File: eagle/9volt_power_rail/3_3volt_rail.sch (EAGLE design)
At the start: 32 parts, among them X1 5566-4, X2 5566-4, X3 5566-4, X4 5566-4, X5 5566-4, X6 5566-4

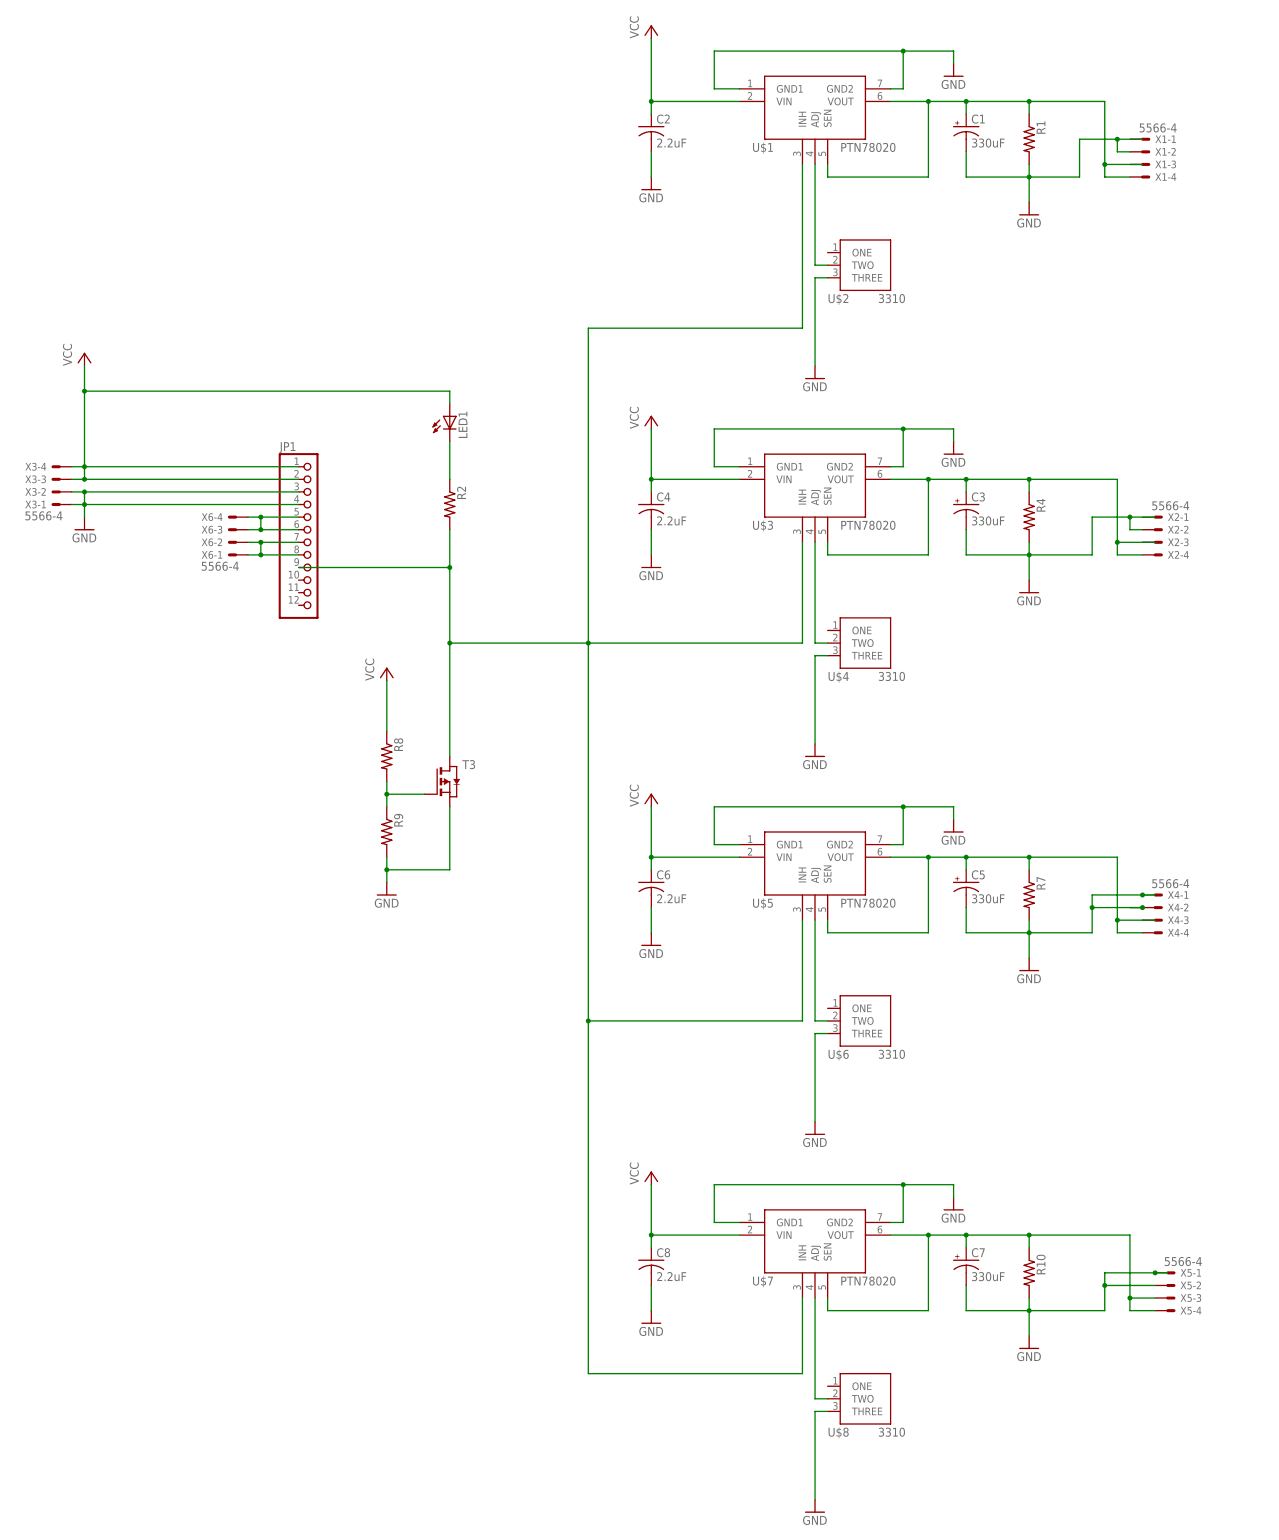
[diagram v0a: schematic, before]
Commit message: moving to lab computer
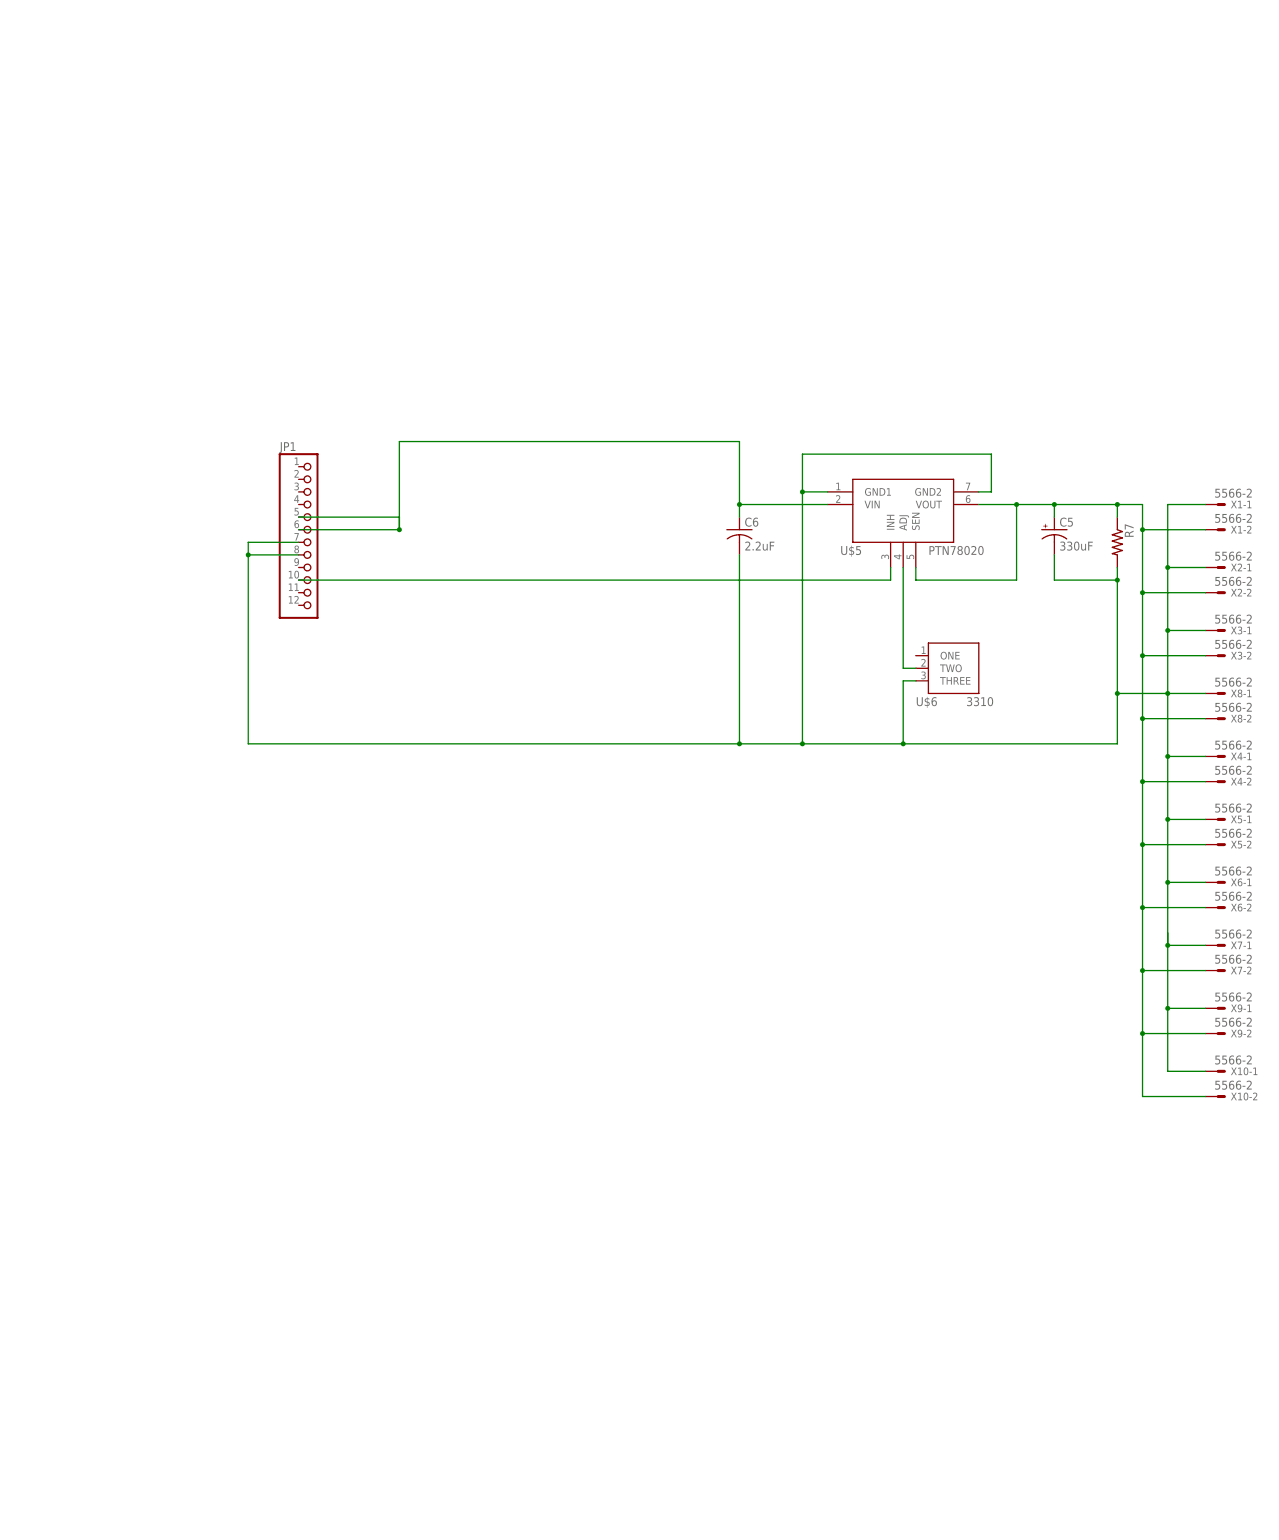
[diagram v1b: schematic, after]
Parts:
- removed C1, C3, C7: 330uF, rcl:CPOL-USE5-10.5
- removed C2, C4, C8: 2.2uF, adafruit:C-USC0805
- removed LED1: (no value), adafruit:LED5MM
- removed R1, R10, R2, R4, R8, R9: (no value), adafruit:R-US_M0805
- removed T3: (no value), zetex:PMOSSOT223
- removed U$1, U$3, U$7: PTH78020-SMD, PTN78020:PTH78020-SMD
- removed U$2, U$4, U$8: 3310-001, 3310-001:3310-001
- added X10, X7, X8, X9: 5566-2, con-molex:5566-2
- X1, X2, X3, X4, X5, X6: value 5566-4 -> 5566-2; device con-molex:5566-4 -> con-molex:5566-2
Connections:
- removed net GND: C1.-, C2.2, C3.-, C4.2, C5.-, C6.2, C7.-, C8.2, JP1.3, JP1.4, R1.2, R10.2, R4.2, R7.2, R9.2, T3.S, U$1.GND1, U$1.GND2, U$2.THREE, U$3.GND1, U$3.GND2, U$4.THREE, U$5.GND1, U$5.GND2, U$6.THREE, U$7.GND1, U$7.GND2, U$8.THREE, X1-2.S, X2-2.S, X3-1.S, X3-2.S, X4-1.S, X4-2.S, X5-1.S, X5-2.S
- removed net N$1: C3.+, R4.1, U$3.SEN, U$3.VOUT, X2-4.S
- removed net N$10: JP1.7, JP1.8, X6-1.S, X6-2.S
- removed net N$12: U$3.ADJ, U$4.TWO
- removed net N$14: R8.2, R9.1, T3.G
- removed net N$2: U$1.ADJ, U$2.TWO
- removed net N$22: U$7.ADJ, U$8.TWO
- removed net N$5: JP1.9, R2.2, T3.D, U$1.INH, U$3.INH, U$5.INH, U$7.INH
- removed net N$6: C5.+, R7.1, U$5.SEN, U$5.VOUT, X4-3.S, X4-4.S
- removed net N$9: C7.+, R10.1, U$7.SEN, U$7.VOUT, X5-3.S, X5-4.S
- removed net VCC: C2.1, C4.1, C6.1, C8.1, JP1.1, JP1.2, LED1.A, R8.1, U$1.VIN, U$3.VIN, U$5.VIN, U$7.VIN, X3-3.S, X3-4.S
- new net N$11: C6.1, JP1.5, JP1.6, U$5.VIN
- net N$3: now also C5.+, R7.1, U$5.SEN, U$5.VOUT, X1-2.S, X10-2.S, X2-2.S, X3-2.S, X4-2.S, X5-2.S, X6-2.S, X7-2.S, X8-2.S, X9-2.S; no longer C1.+, R1.1, U$1.SEN, U$1.VOUT, X1-4.S
- net N$4: now also C5.-, C6.2, JP1.7, JP1.8, R7.2, U$5.GND1, U$5.GND2, U$6.THREE, X1-1.S, X10-1.S, X2-1.S, X3-1.S, X4-1.S, X5-1.S, X6-1.S, X7-1.S, X8-1.S, X9-1.S; no longer LED1.C, R2.1
- net N$7: now also JP1.10, U$5.INH; no longer JP1.5, JP1.6, X6-3.S, X6-4.S
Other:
- moved on the sheet: C5, C6, R7, U$5, U$6, X1-1, X1-2, X2-1, X2-2, X3-1, X3-2, X4-1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
